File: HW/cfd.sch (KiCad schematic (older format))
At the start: 38 parts

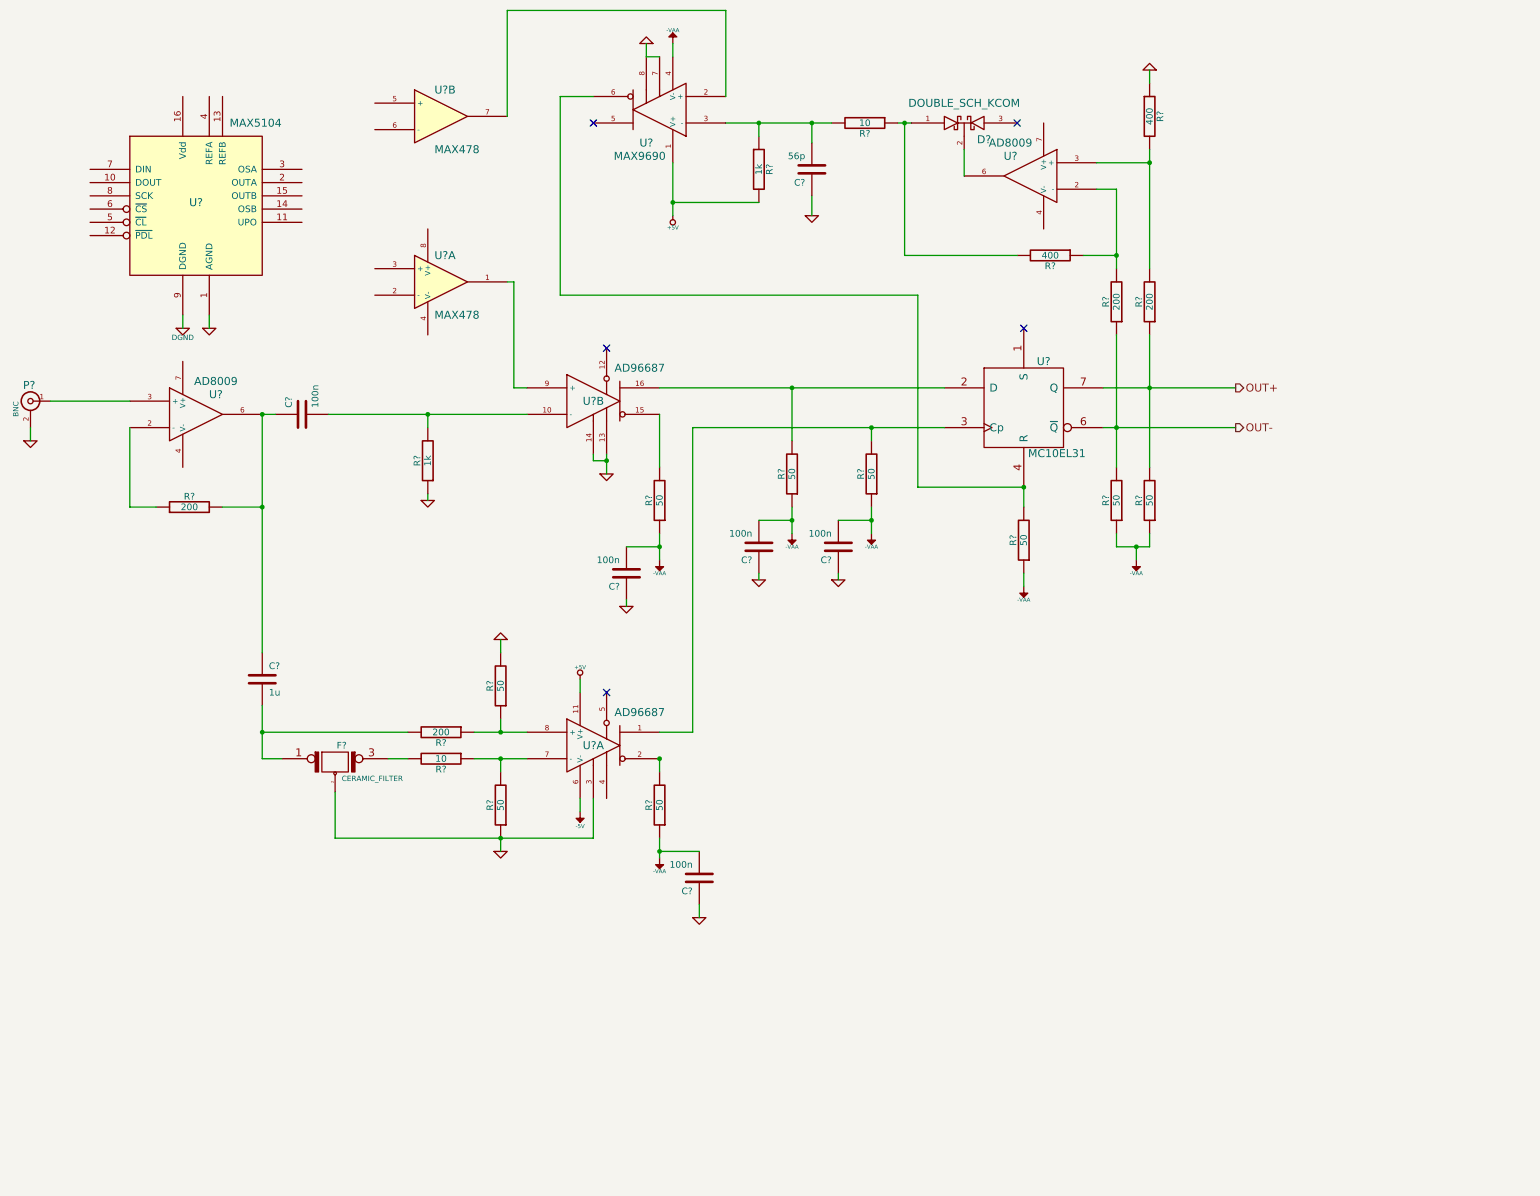
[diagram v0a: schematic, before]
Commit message: Update of CFD
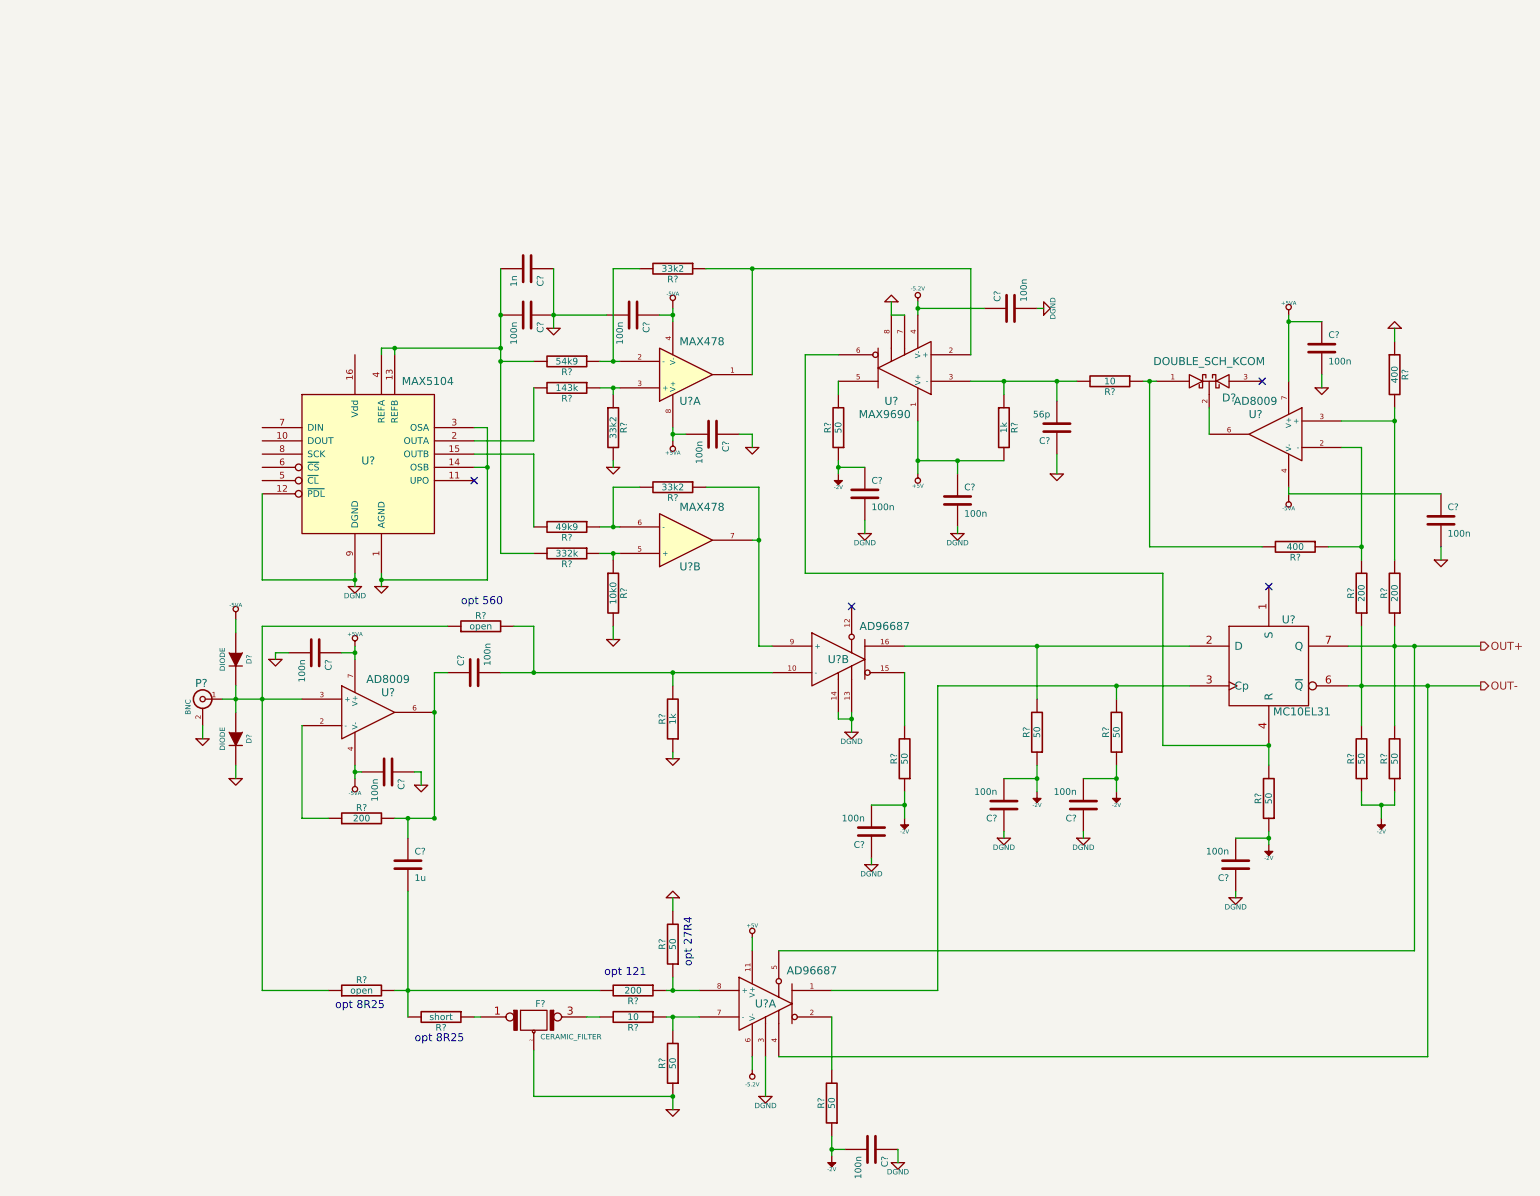
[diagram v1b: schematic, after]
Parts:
- added C? (x11): 100n, symbol C
- added C?: 1n, symbol C
- added D? (x2): DIODE, symbol DIODE
- added R?: 49k9, symbol R
- added R? (x3): 33k2, symbol R
- added R?: 332k, symbol R
- added R?: 10k0, symbol R
- added R?: 50, symbol R
- added R?: 143k, symbol R
- added R?: 54k9, symbol R
- added R? (x2): open, symbol R
- added R?: short, symbol R
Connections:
- net +5V: now also C?.1
- net DGND: now also C?.1, C?.1, C?.1, C?.1, U?.12 (~PDL), U?.13, U?.14, U?.3, C?.1, C?.2, C?.2, C?.2
- net GND: now also U?.14 (OSB), U?.3 (OSA), C?.1, C?.1, C?.1, C?.1, C?.2, C?.2, C?.2, C?.2, D?.2 (K), R?.2, R?.2; no longer C?.1, C?.1, C?.1, C?.1, U?.13, U?.14, U?.3
- net OUT+: now also U?.5
- net OUT-: now also U?.4
- net at P?.1 (In), U?.3 (+): now also D?.1 (A), D?.2 (K), R?.1, R?.1
- net -5VA: now reaches U?.4 (V-)
- net -5VA: now also U?.4 (V-), U?.4 (V-), C?.1, C?.1, C?.2, D?.1 (A)
- net +5VA: now reaches U?.7 (V+)
- net +5VA: now also U?.7 (V+), U?.8 (V+), C?.1, C?.1, C?.2
- net at C?.2, R?.2, U?.10 (-): now also R?.2
- net at U?.9 (+): now also U?.7, R?.1; no longer U?.1
- net at C?.2, R?.2: now also R?.2, R?.2; no longer F?.1 (P1)
- net at U?.2 (+): now also U?.1, R?.1; no longer U?.7
- net at U?.5: now also R?.2
- net at U?.13 (REFB): now also U?.4 (REFA), C?.2, C?.2, R?.2, R?.2
- net at U?.15 (OUTB): now also R?.2
- net at U?.2 (OUTA): now also R?.2
- net -5V renamed -5V2
- net -5V2: now also U?.4 (V-), C?.1
- net -VAA renamed -2V
- net -2V: now also C?.1, C?.2, R?.1; no longer U?.4 (V-)
- new net: F?.1 (P1), R?.1
- new net: R?.1, R?.1, U?.5 (+)
- new net: R?.1, R?.2, U?.6 (-)
- new net: R?.1, R?.2, U?.2 (-)
- new net: R?.1, R?.1, U?.3 (+)
- no-connect marks 5 -> 4
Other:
- note added: "opt 121"
- note added: "opt 27R4"
- note added: "opt 560"
- note added: "opt 8R25"
- moved on the sheet: C?, D?, F?, P?, R?, U?, U?A, U?B
